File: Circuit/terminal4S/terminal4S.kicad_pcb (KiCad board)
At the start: 2 copper layers, 10 parts, among them J1 Conn_01x05_Male, J2 Conn_02x08_Odd_Even, J3 Conn_01x02_Male, U1 4051

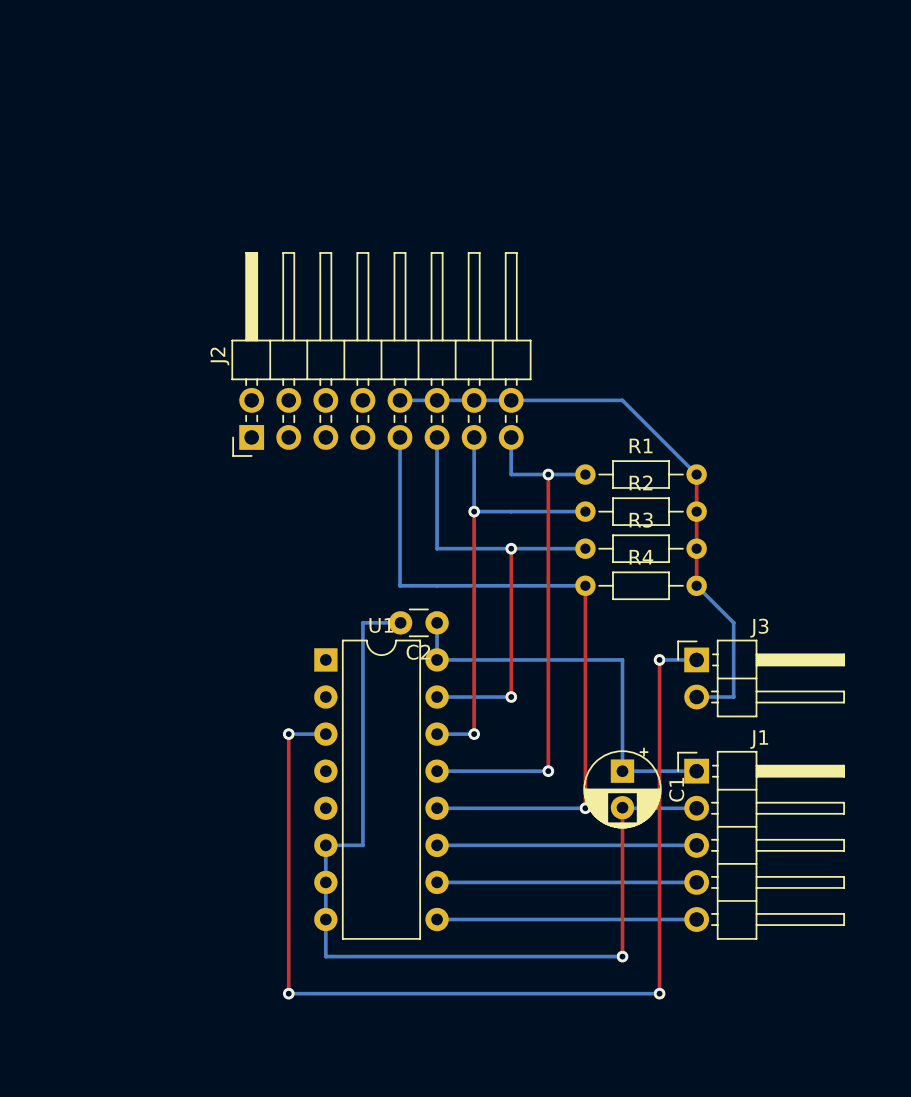
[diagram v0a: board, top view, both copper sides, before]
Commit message: ECM対策
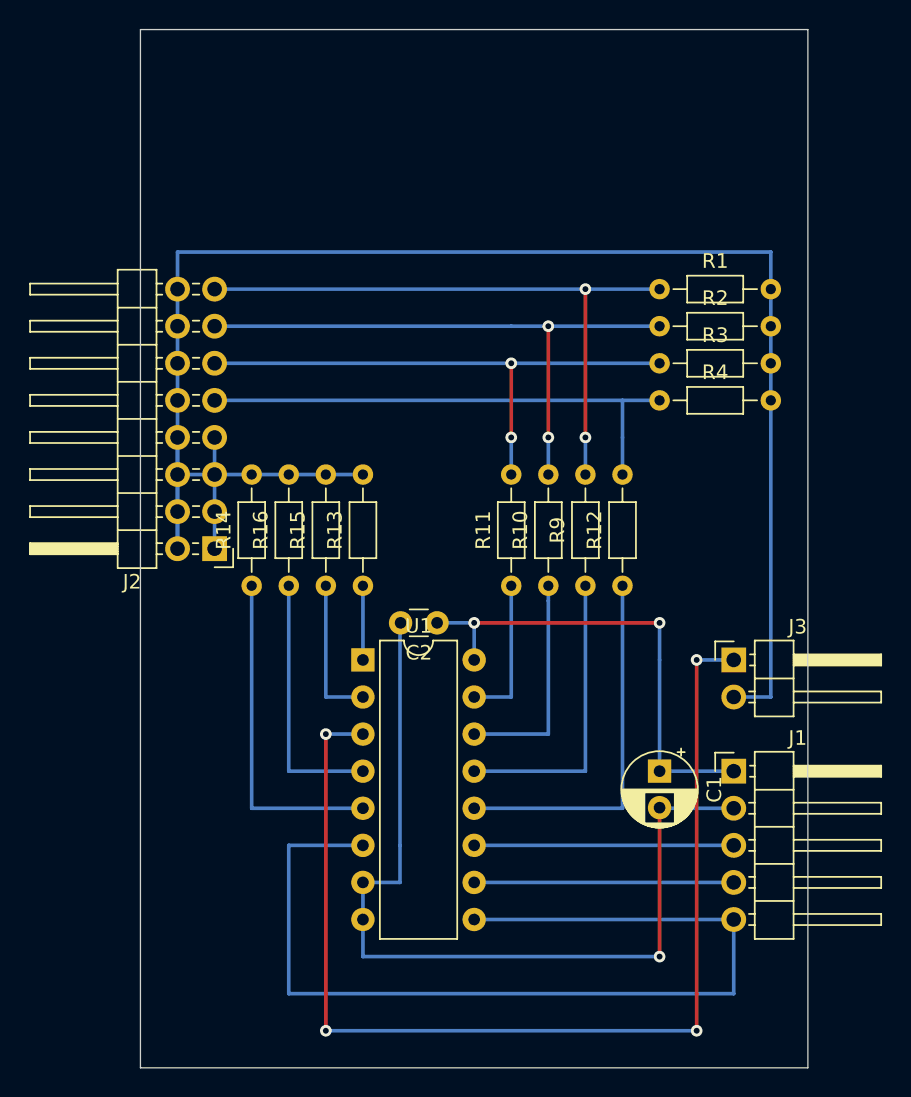
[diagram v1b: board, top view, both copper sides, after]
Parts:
- added R10: 220, Resistor_THT:R_Axial_DIN0204_L3.6mm_D1.6mm_P7.62mm_Horizontal, F.Cu at (132.1, 71.1)
- added R11: 220, Resistor_THT:R_Axial_DIN0204_L3.6mm_D1.6mm_P7.62mm_Horizontal, F.Cu at (129.5, 71.1)
- added R12: 220, Resistor_THT:R_Axial_DIN0204_L3.6mm_D1.6mm_P7.62mm_Horizontal, F.Cu at (137.2, 71.1)
- added R13: 220, Resistor_THT:R_Axial_DIN0204_L3.6mm_D1.6mm_P7.62mm_Horizontal, F.Cu at (119.4, 71.1)
- added R14: 220, Resistor_THT:R_Axial_DIN0204_L3.6mm_D1.6mm_P7.62mm_Horizontal, F.Cu at (111.8, 71.1)
- added R15: 220, Resistor_THT:R_Axial_DIN0204_L3.6mm_D1.6mm_P7.62mm_Horizontal, F.Cu at (116.8, 71.1)
- added R16: 220, Resistor_THT:R_Axial_DIN0204_L3.6mm_D1.6mm_P7.62mm_Horizontal, F.Cu at (114.3, 71.1)
- added R9: 220, Resistor_THT:R_Axial_DIN0204_L3.6mm_D1.6mm_P7.62mm_Horizontal, F.Cu at (134.6, 71.1)
- moved R1 13.7 mm to (139.7, 50.8)
- moved R2 13.7 mm to (139.7, 53.3)
- moved R4 13.7 mm to (139.7, 58.4)
- moved R3 13.7 mm to (139.7, 55.9)
- moved J2 8.03 mm to (109.2, 68.6), turned to 180 degrees
- moved C1 2.54 mm to (139.7, 83.8)
- moved J1 2.54 mm to (144.8, 83.8)
- moved J3 2.54 mm to (144.8, 76.2)
- moved U1 2.54 mm to (119.4, 76.2)
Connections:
- J2 pad 1: (no net) -> Net-(J2-Pad1)
- J2 pad 10: Net-(J2-Pad10) -> Net-(J2-Pad1)
- J2 pad 12: Net-(J2-Pad10) -> Net-(J2-Pad1)
- J2 pad 14: Net-(J2-Pad10) -> Net-(J2-Pad1)
- J2 pad 16: Net-(J2-Pad10) -> Net-(J2-Pad1)
- J2 pad 2: (no net) -> Net-(J2-Pad1)
- J2 pad 3: (no net) -> Net-(J2-Pad1)
- J2 pad 4: (no net) -> Net-(J2-Pad1)
- J2 pad 5: (no net) -> Net-(J2-Pad1)
- J2 pad 6: (no net) -> Net-(J2-Pad1)
- J2 pad 7: (no net) -> Net-(J2-Pad1)
- J2 pad 8: (no net) -> Net-(J2-Pad1)
- J3 pad 2: Net-(J2-Pad10) -> Net-(J2-Pad1)
- R1 pad 2: Net-(J2-Pad10) -> Net-(J2-Pad1)
- R2 pad 2: Net-(J2-Pad10) -> Net-(J2-Pad1)
- R3 pad 2: Net-(J2-Pad10) -> Net-(J2-Pad1)
- R4 pad 2: Net-(J2-Pad10) -> Net-(J2-Pad1)
- U1 pad 1: (no net) -> Net-(R13-Pad1)
- U1 pad 12: Net-(J2-Pad9) -> Net-(R12-Pad1)
- U1 pad 13: Net-(J2-Pad15) -> Net-(R9-Pad1)
- U1 pad 14: Net-(J2-Pad13) -> Net-(R10-Pad1)
- U1 pad 15: Net-(J2-Pad11) -> Net-(R11-Pad1)
- U1 pad 2: (no net) -> Net-(R15-Pad1)
- U1 pad 4: (no net) -> Net-(R16-Pad1)
- U1 pad 5: (no net) -> Net-(R14-Pad1)
- U1 pad 6: GND -> Net-(J1-Pad5)
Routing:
- net Net-(J2-Pad1): track 0.00 -> 121.9 mm
- net Net-(J1-Pad5): track 17.8 -> 68.6 mm
- net Net-(J2-Pad10): track 41.3 -> 0.00 mm
- net Net-(R12-Pad1): track 0.00 -> 25.4 mm
- net Net-(R14-Pad1): track 0.00 -> 22.9 mm
- net Net-(R9-Pad1): track 0.00 -> 20.3 mm
- net Net-(R16-Pad1): track 0.00 -> 17.8 mm
- net Net-(R10-Pad1): track 0.00 -> 15.2 mm
- net Net-(J2-Pad9): track 48.3 -> 35.6 mm, vias 1 -> 0
- net Net-(R15-Pad1): track 0.00 -> 10.2 mm
- net Net-(R11-Pad1): track 0.00 -> 10.2 mm
- net Net-(J2-Pad13): track 30.5 -> 40.6 mm
- net Net-(J2-Pad15): track 35.6 -> 43.2 mm
- net VDD: track 27.9 -> 33.0 mm, vias 0 -> 2
- net Net-(R13-Pad1): track 0.00 -> 5.08 mm
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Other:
- board outline added: 45.7 x 71.1 mm
- board text added: "Akizuki Type C Board (17x27)"
